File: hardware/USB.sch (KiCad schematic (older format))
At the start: 9 parts, among them IC9 FT232RL, J2 USB_A

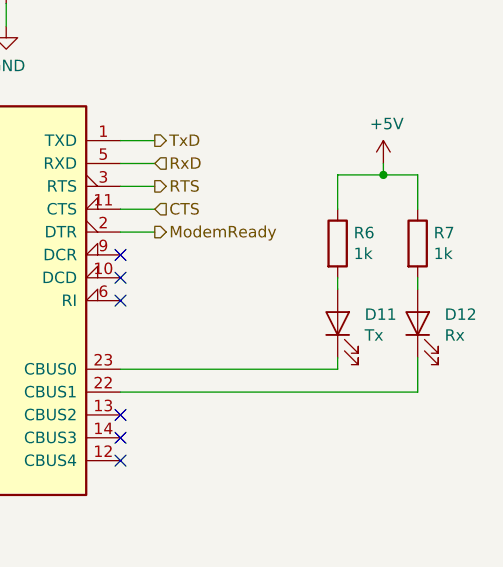
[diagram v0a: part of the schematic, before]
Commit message: Working on layout
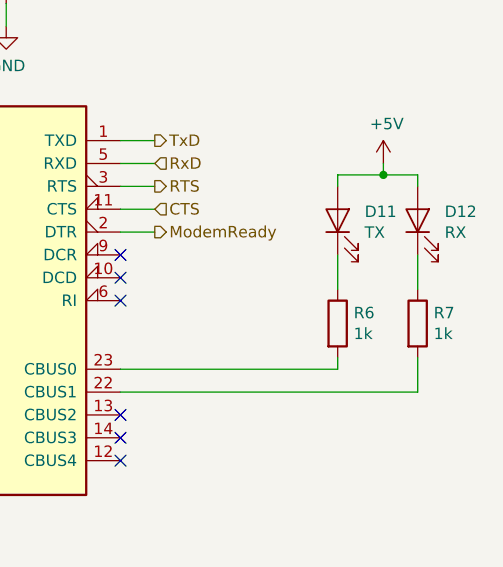
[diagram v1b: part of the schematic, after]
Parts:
- D11: value Tx -> TX
- D12: value Rx -> RX
- J2: value USB_A -> SERIAL; Mfr. (none) -> Wurth Elektronik; Mfr. No. (none) -> 629105150521; Mouser (none) -> 710-629105150521
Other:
- moved on the sheet: D11, D12, R6, R7
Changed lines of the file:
@@
 EESchema Schematic File Version 4
-LIBS:Sweet 6502 Computer-cache
+LIBS:Retro PC-cache
 EELAYER 30 0
 EELAYER END
@@
 AR Path="/5E9064F2/5E95D1DF" Ref="J2"  Part="1"
 F 0 "J2" H 2970 3347 50  0000 R CNN
-F 1 "USB_A" H 2970 3438 50  0000 R CNN
+F 1 "SERIAL" H 2970 3438 50  0000 R CNN
 F 2 "Connector_USB:USB_Micro-B_Wuerth_629105150521" H 3350 3400 50  0001 C CNN
 F 3 "https://www.belfuse.com/resources/datasheets/stewartconnector/ds-stw-usb-2.0-and-3.0-connectors.pdf" H 3350 3400 50  0001 C CNN
-F 4 "" H 3200 3450 50  0001 C CNN "Mfr."
-F 5 "" H 3200 3450 50  0001 C CNN "Mfr. No."
-F 6 "" H 3200 3450 50  0001 C CNN "Mouser"
+F 4 "Wurth Elektronik" H 3200 3450 50  0001 C CNN "Mfr."
+F 5 "629105150521" H 3200 3450 50  0001 C CNN "Mfr. No."
+F 6 "710-629105150521" H 3200 3450 50  0001 C CNN "Mouser"
 	1    3200 3450
 	1    0    0    -1
@@
 L Device:LED D?
 U 1 1 5E95D1E6
-P 7400 3950
+P 7400 3500
 AR Path="/5E95D1E6" Ref="D?"  Part="1"
 AR Path="/5E9064F2/5E95D1E6" Ref="D11"  Part="1"
-F 0 "D11" V 7439 3832 50  0000 R CNN
-F 1 "Tx" V 7348 3832 50  0000 R CNN
-F 2 "LED_SMD:LED_0805_2012Metric" H 7400 3950 50  0001 C CNN
-F 3 "https://www.mouser.de/datasheet/2/216/apt2012pyw-1173287.pdf" H 7400 3950 50  0001 C CNN
-F 4 "Kingbright" H 7400 3950 50  0001 C CNN "Mfr."
-F 5 "APT2012PYW" H 7400 3950 50  0001 C CNN "Mfr. No."
-F 6 "604-APT2012PYW" H 7400 3950 50  0001 C CNN "Mouser"
-	1    7400 3950
+F 0 "D11" V 7439 3382 50  0000 R CNN
+F 1 "TX" V 7348 3382 50  0000 R CNN
+F 2 "LED_SMD:LED_0805_2012Metric" H 7400 3500 50  0001 C CNN
+F 3 "https://www.mouser.de/datasheet/2/216/apt2012pyw-1173287.pdf" H 7400 3500 50  0001 C CNN
+F 4 "Kingbright" H 7400 3500 50  0001 C CNN "Mfr."
+F 5 "APT2012PYW" H 7400 3500 50  0001 C CNN "Mfr. No."
+F 6 "604-APT2012PYW" H 7400 3500 50  0001 C CNN "Mouser"
+	1    7400 3500
 	0    -1   -1   0
 $EndComp
@@
 L Device:R R?
 U 1 1 5E95D1EC
-P 7400 3600
+P 7400 3950
 AR Path="/5E95D1EC" Ref="R?"  Part="1"
 AR Path="/5E9064F2/5E95D1EC" Ref="R6"  Part="1"
-F 0 "R6" H 7470 3646 50  0000 L CNN
-F 1 "1k" H 7470 3555 50  0000 L CNN
-F 2 "Resistor_SMD:R_0805_2012Metric" V 7330 3600 50  0001 C CNN
-F 3 "~" H 7400 3600 50  0001 C CNN
-F 4 "Vishay / Dale" H 7400 3600 50  0001 C CNN "Mfr."
-F 5 "CRCW08051K00FKEAC" H 7400 3600 50  0001 C CNN "Mfr. No."
-F 6 "71-CRCW08051K00FKEAC" H 7400 3600 50  0001 C CNN "Mouser"
-	1    7400 3600
+F 0 "R6" H 7470 3996 50  0000 L CNN
+F 1 "1k" H 7470 3905 50  0000 L CNN
+F 2 "Resistor_SMD:R_0805_2012Metric" V 7330 3950 50  0001 C CNN
+F 3 "https://www.mouser.de/datasheet/2/427/crcwce3-1223726.pdf" H 7400 3950 50  0001 C CNN
+F 4 "Vishay / Dale" H 7400 3950 50  0001 C CNN "Mfr."
+F 5 "CRCW08051K00FKEAC" H 7400 3950 50  0001 C CNN "Mfr. No."
+F 6 "71-CRCW08051K00FKEAC" H 7400 3950 50  0001 C CNN "Mouser"
+	1    7400 3950
 	1    0    0    -1
 $EndComp
@@
 L Device:R R?
 U 1 1 5E95D1F2
-P 7750 3600
+P 7750 3950
 AR Path="/5E95D1F2" Ref="R?"  Part="1"
 AR Path="/5E9064F2/5E95D1F2" Ref="R7"  Part="1"
-F 0 "R7" H 7820 3646 50  0000 L CNN
-F 1 "1k" H 7820 3555 50  0000 L CNN
-F 2 "Resistor_SMD:R_0805_2012Metric" V 7680 3600 50  0001 C CNN
-F 3 "~" H 7750 3600 50  0001 C CNN
-F 4 "Vishay / Dale" H 7750 3600 50  0001 C CNN "Mfr."
-F 5 "CRCW08051K00FKEAC" H 7750 3600 50  0001 C CNN "Mfr. No."
-F 6 "71-CRCW08051K00FKEAC" H 7750 3600 50  0001 C CNN "Mouser"
-	1    7750 3600
+F 0 "R7" H 7820 3996 50  0000 L CNN
+F 1 "1k" H 7820 3905 50  0000 L CNN
+F 2 "Resistor_SMD:R_0805_2012Metric" V 7680 3950 50  0001 C CNN
+F 3 "https://www.mouser.de/datasheet/2/427/crcwce3-1223726.pdf" H 7750 3950 50  0001 C CNN
+F 4 "Vishay / Dale" H 7750 3950 50  0001 C CNN "Mfr."
+F 5 "CRCW08051K00FKEAC" H 7750 3950 50  0001 C CNN "Mfr. No."
+F 6 "71-CRCW08051K00FKEAC" H 7750 3950 50  0001 C CNN "Mouser"
+	1    7750 3950
 	1    0    0    -1
 $EndComp
@@
 L Device:LED D?
 U 1 1 5E95D1F8
-P 7750 3950
+P 7750 3500
 AR Path="/5E95D1F8" Ref="D?"  Part="1"
 AR Path="/5E9064F2/5E95D1F8" Ref="D12"  Part="1"
-F 0 "D12" V 7789 3832 50  0000 R CNN
-F 1 "Rx" V 7698 3832 50  0000 R CNN
-F 2 "LED_SMD:LED_0805_2012Metric" H 7750 3950 50  0001 C CNN
-F 3 "https://www.mouser.de/datasheet/2/216/apt2012pgw-1173286.pdf" H 7750 3950 50  0001 C CNN
-F 4 "Kingbright" H 7750 3950 50  0001 C CNN "Mfr."
-F 5 "APT2012PGW" H 7750 3950 50  0001 C CNN "Mfr. No."
-F 6 "604-APT2012PGW" H 7750 3950 50  0001 C CNN "Mouser"
-	1    7750 3950
+F 0 "D12" V 7789 3382 50  0000 R CNN
+F 1 "RX" V 7698 3382 50  0000 R CNN
+F 2 "LED_SMD:LED_0805_2012Metric" H 7750 3500 50  0001 C CNN
+F 3 "https://www.mouser.de/datasheet/2/216/apt2012pgw-1173286.pdf" H 7750 3500 50  0001 C CNN
+F 4 "Kingbright" H 7750 3500 50  0001 C CNN "Mfr."
+F 5 "APT2012PGW" H 7750 3500 50  0001 C CNN "Mfr. No."
+F 6 "604-APT2012PGW" H 7750 3500 50  0001 C CNN "Mouser"
+	1    7750 3500
 	0    -1   -1   0
 $EndComp
@@
 F 1 "100nF" H 4515 3105 50  0000 L CNN
 F 2 "Capacitor_SMD:C_0805_2012Metric" H 4438 3000 50  0001 C CNN
-F 3 "~" H 4400 3150 50  0001 C CNN
+F 3 "https://www.mouser.de/datasheet/2/212/KEM_C1002_X7R_SMD-1102033.pdf" H 4400 3150 50  0001 C CNN
 F 4 "KEMET" H 4400 3150 50  0001 C CNN "Mfr."
 F 5 "C0805C104K5RACTU" H 4400 3150 50  0001 C CNN "Mfr. No."
@@
 	7600 3300 7400 3300
 Wire Wire Line
-	7400 3300 7400 3450
-Wire Wire Line
 	7600 3300 7750 3300
-Wire Wire Line
-	7750 3300 7750 3450
 Connection ~ 7600 3300
 Wire Wire Line
-	7750 3750 7750 3800
-Wire Wire Line
-	7400 3750 7400 3800
-Wire Wire Line
 	6450 4150 7400 4150
 Wire Wire Line
-	7400 4150 7400 4100
-Wire Wire Line
 	6450 4250 7750 4250
 Wire Wire Line
-	7750 4250 7750 4100
+	7750 3800 7750 3650
 Wire Wire Line
 	4750 3850 4850 3850
@@
 F 1 "100nF" H 5265 2355 50  0000 L CNN
 F 2 "Capacitor_SMD:C_0805_2012Metric" H 5188 2250 50  0001 C CNN
-F 3 "~" H 5150 2400 50  0001 C CNN
+F 3 "https://www.mouser.de/datasheet/2/212/KEM_C1002_X7R_SMD-1102033.pdf" H 5150 2400 50  0001 C CNN
 F 4 "KEMET" H 5150 2400 50  0001 C CNN "Mfr."
 F 5 "C0805C104K5RACTU" H 5150 2400 50  0001 C CNN "Mfr. No."
@@
 F 1 "100nF" H 6065 2355 50  0000 L CNN
 F 2 "Capacitor_SMD:C_0805_2012Metric" H 5988 2250 50  0001 C CNN
-F 3 "~" H 5950 2400 50  0001 C CNN
+F 3 "https://www.mouser.de/datasheet/2/212/KEM_C1002_X7R_SMD-1102033.pdf" H 5950 2400 50  0001 C CNN
 F 4 "KEMET" H 5950 2400 50  0001 C CNN "Mfr."
 F 5 "C0805C104K5RACTU" H 5950 2400 50  0001 C CNN "Mfr. No."
@@
 	5750 2000 5750 2100
 Connection ~ 5750 2100
+Wire Wire Line
+	7400 4100 7400 4150
+Wire Wire Line
+	7750 4100 7750 4250
+Wire Wire Line
+	7400 3650 7400 3800
+Wire Wire Line
+	7400 3350 7400 3300
+Wire Wire Line
+	7750 3350 7750 3300
 $EndSCHEMATC
